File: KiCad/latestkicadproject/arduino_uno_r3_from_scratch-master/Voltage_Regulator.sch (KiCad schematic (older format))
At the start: 8 parts, among them IC1 MC33269ST-5.OT3, U2 LP2985-33DBVR, X2 DG3XX-02-3.5

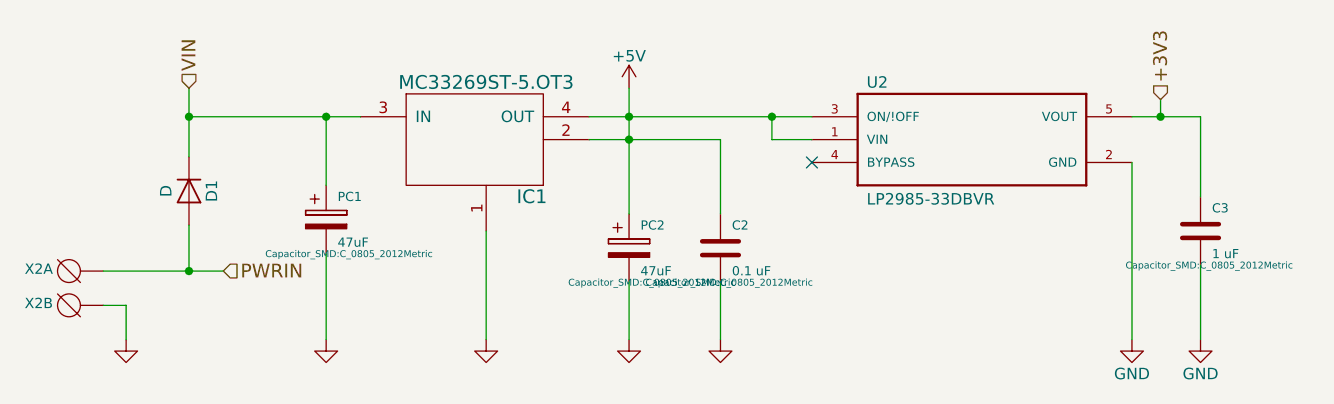
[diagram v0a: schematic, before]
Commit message: pcb routing
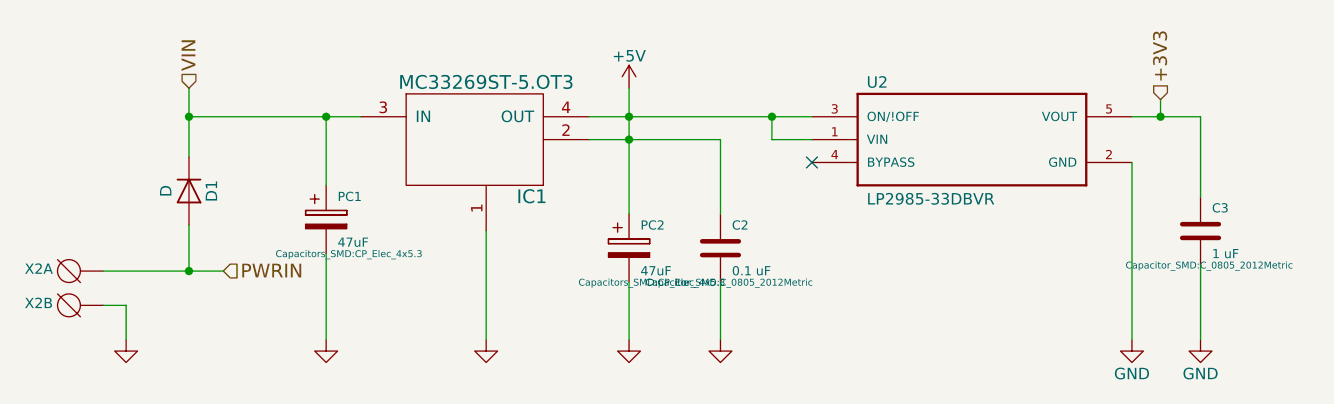
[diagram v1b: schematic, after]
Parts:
- D1: footprint Diodes_SMD:D_0805 -> Diodes_SMD:D_MicroMELF_Hadsoldering
- PC1, PC2: footprint Capacitor_SMD:C_0805_2012Metric -> Capacitors_SMD:CP_Elec_4x5.3
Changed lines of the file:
@@
 LIBS:LP2985-33DBVR
 LIBS:degson
+LIBS:PHT6NQ10T_135
 EELAYER 25 0
 EELAYER END
@@
 F 0 "PC1" H 5075 3975 40  0000 L CNN
 F 1 "47uF" H 5075 3775 40  0000 L CNN
-F 2 "Capacitor_SMD:C_0805_2012Metric" H 5125 3725 30  0000 C CNN
+F 2 "Capacitors_SMD:CP_Elec_4x5.3" H 5125 3725 30  0000 C CNN
 F 3 "http://images.ihscontent.net/vipimages/VipMasterIC/IC/BEYS/BEYSS04513/BEYSS04513-1.pdf" H 5025 3875 300 0001 C CNN
 F 4 "CAPACITOR, ALUMINUM ELECTROLYTIC, NON SOLID, POLARIZED, 50 V, 47 uF, SURFACE MOUNT, 3131, CHIP, ROHS COMPLIANT" H 5025 3875 60  0001 C CNN "Characteristics"
@@
 F 0 "PC2" H 6400 4100 40  0000 L CNN
 F 1 "47uF" H 6400 3900 40  0000 L CNN
-F 2 "Capacitor_SMD:C_0805_2012Metric" H 6450 3850 30  0000 C CNN
+F 2 "Capacitors_SMD:CP_Elec_4x5.3" H 6450 3850 30  0000 C CNN
 F 3 "http://images.ihscontent.net/vipimages/VipMasterIC/IC/BEYS/BEYSS04513/BEYSS04513-1.pdf" H 6350 4000 300 0001 C CNN
 F 4 "CAPACITOR, ALUMINUM ELECTROLYTIC, NON SOLID, POLARIZED, 50 V, 47 uF, SURFACE MOUNT, 3131, CHIP, ROHS COMPLIANT" H 6350 4000 60  0001 C CNN "Characteristics"
@@
 F 0 "D1" H 4425 3850 50  0000 C CNN
 F 1 "D" H 4425 3650 50  0000 C CNN
-F 2 "Diodes_SMD:D_0805" H 4425 3750 50  0001 C CNN
+F 2 "Diodes_SMD:D_MicroMELF_Hadsoldering" H 4425 3750 50  0001 C CNN
 F 3 "" H 4425 3750 50  0001 C CNN
 	1    4425 3750

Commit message: PCB routing v1
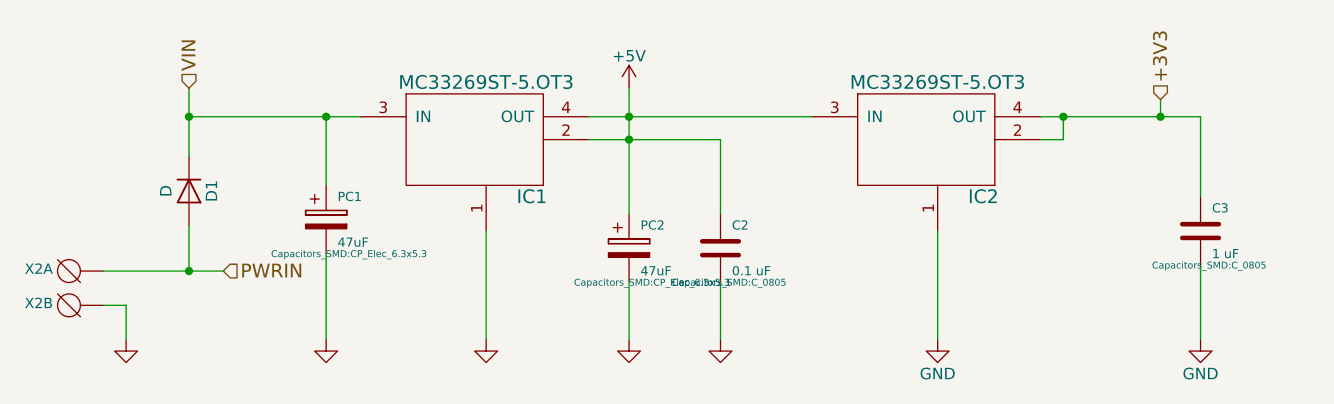
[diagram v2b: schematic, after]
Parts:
- removed U2: LP2985-33DBVR, LP2985-33DBVR:SOT95P280X145-5N, symbol LP2985-33DBVR
- added IC2: MC33269ST-5.OT3, MC33269ST-3.3T3G:SOT230P700X175-4N, symbol MC33269ST-5.OT3
- C2, C3: footprint Capacitor_SMD:C_0805_2012Metric -> Capacitors_SMD:C_0805
- PC1, PC2: footprint Capacitors_SMD:CP_Elec_4x5.3 -> Capacitors_SMD:CP_Elec_6.3x5.3
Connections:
- net +3V3: now also IC2.2, IC2.4 (OUT)
- net +5V: now also IC2.3 (IN)
- net GND: now also IC2.1
- no-connect marks 1 -> 0
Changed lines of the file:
@@
 LIBS:degson
 LIBS:PHT6NQ10T_135
+LIBS:L298P
 EELAYER 25 0
 EELAYER END
@@
 F 0 "PC1" H 5075 3975 40  0000 L CNN
 F 1 "47uF" H 5075 3775 40  0000 L CNN
-F 2 "Capacitors_SMD:CP_Elec_4x5.3" H 5125 3725 30  0000 C CNN
+F 2 "Capacitors_SMD:CP_Elec_6.3x5.3" H 5125 3725 30  0000 C CNN
 F 3 "http://images.ihscontent.net/vipimages/VipMasterIC/IC/BEYS/BEYSS04513/BEYSS04513-1.pdf" H 5025 3875 300 0001 C CNN
 F 4 "CAPACITOR, ALUMINUM ELECTROLYTIC, NON SOLID, POLARIZED, 50 V, 47 uF, SURFACE MOUNT, 3131, CHIP, ROHS COMPLIANT" H 5025 3875 60  0001 C CNN "Characteristics"
@@
 F 0 "C2" H 6800 4100 40  0000 L CNN
 F 1 "0.1 uF" H 6800 3900 40  0000 L CNN
-F 2 "Capacitor_SMD:C_0805_2012Metric" H 6788 3850 30  0000 C CNN
+F 2 "Capacitors_SMD:C_0805" H 6788 3850 30  0000 C CNN
 F 3 "http://images.ihscontent.net/vipimages/VipMasterIC/IC/KEME/KEMES10043/KEMES10043-1.pdf" H 6750 4000 60  0001 C CNN
 F 4 "CAPACITOR, CERAMIC, MULTILAYER, 100 V, X7R, 0.1 uF, SURFACE MOUNT, 0805, CHIP, ROHS COMPLIANT" H 6750 4000 60  0001 C CNN "Characteristics"
@@
 F 0 "PC2" H 6400 4100 40  0000 L CNN
 F 1 "47uF" H 6400 3900 40  0000 L CNN
-F 2 "Capacitors_SMD:CP_Elec_4x5.3" H 6450 3850 30  0000 C CNN
+F 2 "Capacitors_SMD:CP_Elec_6.3x5.3" H 6450 3850 30  0000 C CNN
 F 3 "http://images.ihscontent.net/vipimages/VipMasterIC/IC/BEYS/BEYSS04513/BEYSS04513-1.pdf" H 6350 4000 300 0001 C CNN
 F 4 "CAPACITOR, ALUMINUM ELECTROLYTIC, NON SOLID, POLARIZED, 50 V, 47 uF, SURFACE MOUNT, 3131, CHIP, ROHS COMPLIANT" H 6350 4000 60  0001 C CNN "Characteristics"
@@
 Wire Wire Line
 	6750 3525 6750 3850
-Connection ~ 6975 3425
 $Comp
 L GND #PWR06
 U 1 1 5AA01DB9
-P 8550 4400
-F 0 "#PWR06" H 8550 4150 50  0001 C CNN
-F 1 "GND" H 8550 4250 50  0000 C CNN
-F 2 "" H 8550 4400 50  0001 C CNN
-F 3 "" H 8550 4400 50  0001 C CNN
-	1    8550 4400
-	1    0    0    -1
-$EndComp
-Wire Wire Line
-	8550 3625 8550 4400
+P 7700 4400
+F 0 "#PWR06" H 7700 4150 50  0001 C CNN
+F 1 "GND" H 7700 4250 50  0000 C CNN
+F 2 "" H 7700 4400 50  0001 C CNN
+F 3 "" H 7700 4400 50  0001 C CNN
+	1    7700 4400
+	1    0    0    -1
+$EndComp
 $Comp
 L C C3
@@
 F 0 "C3" H 8900 4025 40  0000 L CNN
 F 1 "1 uF" H 8900 3825 40  0000 L CNN
-F 2 "Capacitor_SMD:C_0805_2012Metric" H 8888 3775 30  0000 C CNN
+F 2 "Capacitors_SMD:C_0805" H 8888 3775 30  0000 C CNN
 F 3 "http://images.ihscontent.net/vipimages/VipMasterIC/IC/KEME/KEMES10043/KEMES10043-1.pdf" H 8850 3925 60  0001 C CNN
 F 4 "CAPACITOR, CERAMIC, MULTILAYER, 100 V, X7R, 0.1 uF, SURFACE MOUNT, 0805, CHIP, ROHS COMPLIANT" H 8850 3925 60  0001 C CNN "Characteristics"
@@
 $EndComp
 Wire Wire Line
-	8550 3425 8850 3425
+	8150 3425 8850 3425
 Wire Wire Line
 	8850 3425 8850 3775
@@
 Text HLabel 8675 3350 1    60   Input ~ 0
 +3V3
-Wire Wire Line
-	6975 3425 6975 3525
-Wire Wire Line
-	6975 3525 7150 3525
-$Comp
-L LP2985-33DBVR U2
-U 1 1 5AA06B18
-P 7850 3525
-F 0 "U2" H 7389 3746 50  0000 L BNN
-F 1 "LP2985-33DBVR" H 7389 3235 50  0000 L BNN
-F 2 "LP2985-33DBVR:SOT95P280X145-5N" H 7850 3525 50  0001 L BNN
-F 3 "Good" H 7850 3525 50  0001 L BNN
-F 4 "Texas Instruments" H 7850 3525 50  0001 L BNN "Field4"
-F 5 "IC REG LINEAR 3.3V 150MA SOT23-5" H 7850 3525 50  0001 L BNN "Field5"
-F 6 "0.34 USD" H 7850 3525 50  0001 L BNN "Field6"
-F 7 "SOT-23-5 Texas Instruments" H 7850 3525 50  0001 L BNN "Field7"
-F 8 "LP2985-33DBVR" H 7850 3525 50  0001 L BNN "Field8"
-	1    7850 3525
-	1    0    0    -1
-$EndComp
-NoConn ~ 7150 3625
 Wire Wire Line
 	4150 4250 4150 4400
@@
 	-1   0    0    1
 $EndComp
+$Comp
+L MC33269ST-5.OT3 IC2
+U 1 1 5AB3045E
+P 7700 3525
+F 0 "IC2" H 7900 3275 60  0000 C CNN
+F 1 "MC33269ST-5.OT3" H 7700 3775 60  0000 C CNN
+F 2 "MC33269ST-3.3T3G:SOT230P700X175-4N" H 7350 3425 60  0001 C CNN
+F 3 "" H 7350 3425 60  0001 C CNN
+	1    7700 3525
+	1    0    0    -1
+$EndComp
+Wire Wire Line
+	7700 3925 7700 4400
+Wire Wire Line
+	8150 3525 8250 3525
+Wire Wire Line
+	8250 3525 8250 3425
+Connection ~ 8250 3425
 $EndSCHEMATC
